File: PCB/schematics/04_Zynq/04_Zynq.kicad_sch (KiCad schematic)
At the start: 0 parts

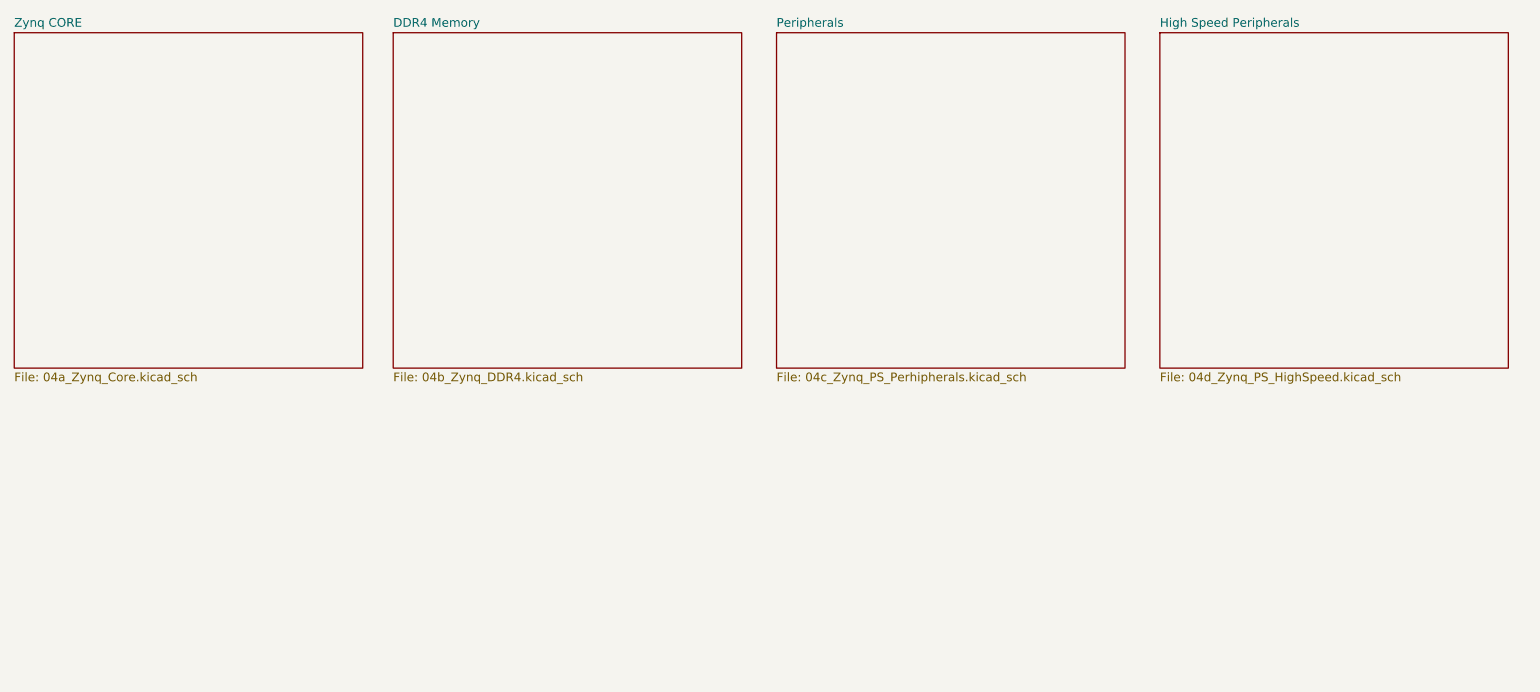
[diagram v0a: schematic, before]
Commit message: feat: Section 4 Done
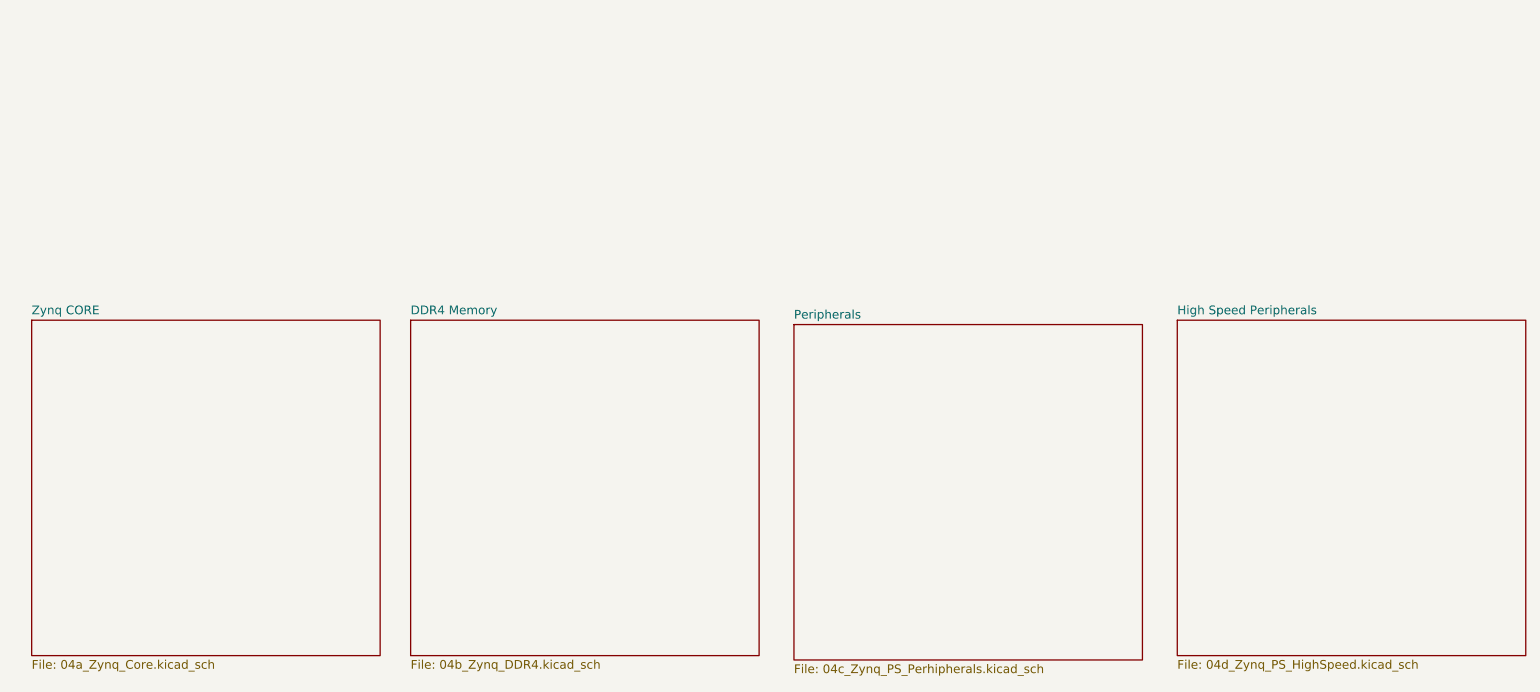
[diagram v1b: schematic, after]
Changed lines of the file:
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@@
 	(generator "eeschema")
 	(generator_version "10.0")
-	(paper "User" 841 800)
+	(paper "A4")
 	(sheet
-		(at 200.66 33.02)
+		(at 203.2 74.93)
 		(size 50.8 48.895)
 		(exclude_from_sim no)
@@
 		)
 		(property "Sheetname" "High Speed Peripherals"
-			(at 200.66 32.3084 0)
+			(at 203.2 74.2184 0)
 			(show_name no)
 			(do_not_autoplace no)
@@
 		)
 		(property "Sheetfile" "04d_Zynq_PS_HighSpeed.kicad_sch"
-			(at 200.66 82.4996 0)
+			(at 203.2 124.4096 0)
 			(show_name no)
 			(do_not_autoplace no)
@@
 					(page "9")
 				)
+				(path "/f4f7837f-dd80-4f77-b150-4534de1c10d6/54437adb-84e2-431a-8017-9277896bf257"
+					(page "13")
+				)
 			)
 		)
 	)
 	(sheet
-		(at 144.78 33.02)
+		(at 147.32 75.565)
 		(size 50.8 48.895)
 		(exclude_from_sim no)
@@
 		)
 		(property "Sheetname" "Peripherals"
-			(at 144.78 32.3084 0)
+			(at 147.32 74.8534 0)
 			(show_name no)
 			(do_not_autoplace no)
@@
 		)
 		(property "Sheetfile" "04c_Zynq_PS_Perhipherals.kicad_sch"
-			(at 144.78 82.4996 0)
+			(at 147.32 125.0446 0)
 			(show_name no)
 			(do_not_autoplace no)
@@
 					(page "8")
 				)
+				(path "/f4f7837f-dd80-4f77-b150-4534de1c10d6/54437adb-84e2-431a-8017-9277896bf257"
+					(page "12")
+				)
 			)
 		)
 	)
 	(sheet
-		(at 88.9 33.02)
+		(at 91.44 74.93)
 		(size 50.8 48.895)
 		(exclude_from_sim no)
@@
 		)
 		(property "Sheetname" "DDR4 Memory"
-			(at 88.9 32.3084 0)
+			(at 91.44 74.2184 0)
 			(show_name no)
 			(do_not_autoplace no)
@@
 		)
 		(property "Sheetfile" "04b_Zynq_DDR4.kicad_sch"
-			(at 88.9 82.4996 0)
+			(at 91.44 124.4096 0)
 			(show_name no)
 			(do_not_autoplace no)
@@
 					(page "7")
 				)
+				(path "/f4f7837f-dd80-4f77-b150-4534de1c10d6/54437adb-84e2-431a-8017-9277896bf257"
+					(page "14")
+				)
 			)
 		)
 	)
 	(sheet
-		(at 33.655 33.02)
+		(at 36.195 74.93)
 		(size 50.8 48.895)
 		(exclude_from_sim no)
@@
 		)
 		(property "Sheetname" "Zynq CORE"
-			(at 33.655 32.3084 0)
+			(at 36.195 74.2184 0)
 			(show_name no)
 			(do_not_autoplace no)
@@
 		)
 		(property "Sheetfile" "04a_Zynq_Core.kicad_sch"
-			(at 33.655 82.4996 0)
+			(at 36.195 124.4096 0)
 			(show_name no)
 			(do_not_autoplace no)
@@
 					(page "6")
 				)
+				(path "/f4f7837f-dd80-4f77-b150-4534de1c10d6/54437adb-84e2-431a-8017-9277896bf257"
+					(page "11")
+				)
 			)
